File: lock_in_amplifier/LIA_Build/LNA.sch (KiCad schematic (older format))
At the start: 45 parts, among them J17 RF_Shield_One_Piece, J38 RF_Shield_One_Piece, U6 lmp7721, U7 LM833, U8 AD8429

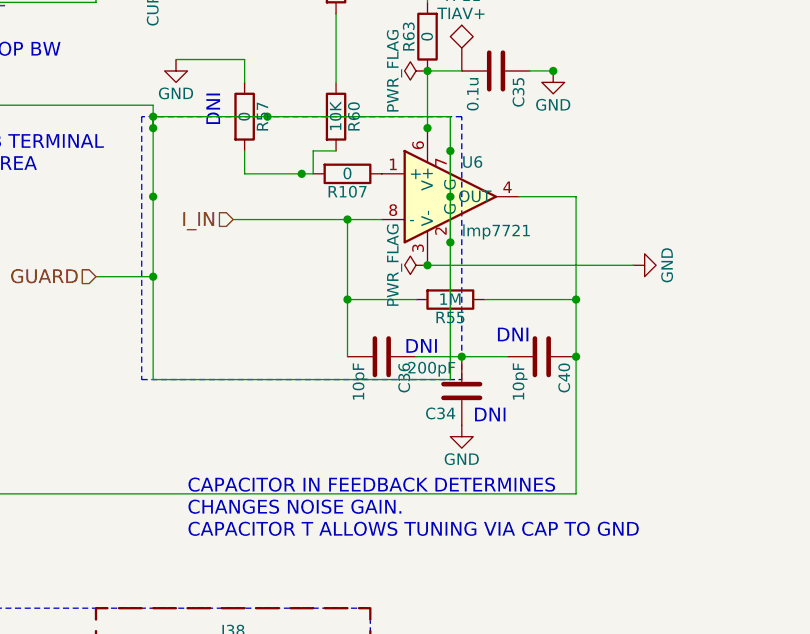
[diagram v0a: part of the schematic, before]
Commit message: adressing comments - fets
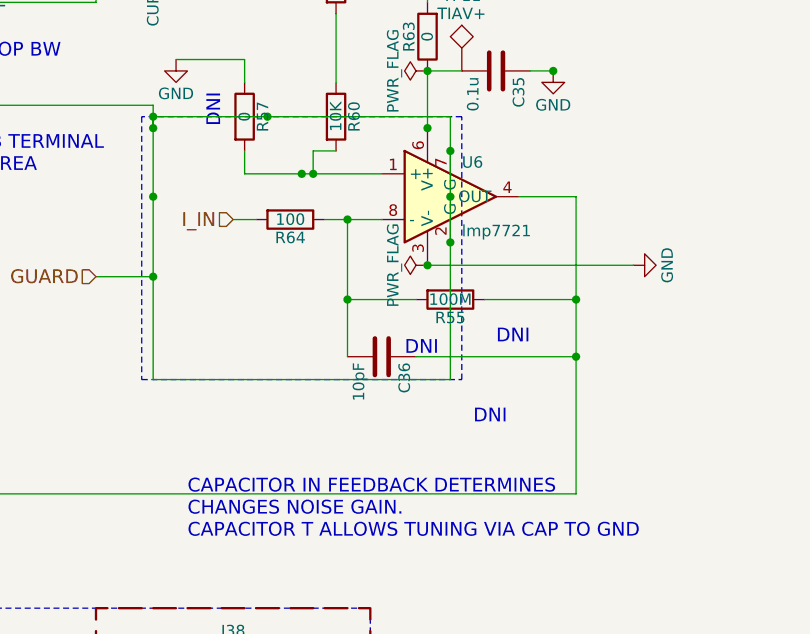
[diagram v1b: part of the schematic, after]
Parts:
- removed C34: 200pF, Capacitors_SMD:C_0805, symbol C
- removed C40: 10pF, Capacitors_SMD:C_0805, symbol C
- removed R107: 0, Resistors_SMD:R_0805, symbol R
- added R64: 100, Resistors_SMD:R_0805, symbol R
- R55: value 1M -> 100M
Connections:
- net I_IN: now also R64.2; no longer C36.2, R55.2, U6.8 (-)
- net at R55.1, S4.1 (B1), TP13.1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: now also C36.1
- net at R57.2, R60.2: now also U6.1 (+)
- new net: C36.2, R55.2, R64.1, U6.8 (-)
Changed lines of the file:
@@
 LIBS:contrib
 LIBS:valves
+LIBS:ada2200
 LIBS:LIA-cache
-LIBS:LNA_test-cache
 EELAYER 25 0
 EELAYER END
 $Descr USLetter 11000 8500
 encoding utf-8
-Sheet 3 3
+Sheet 3 6
 Title "LNA AND TRANSIMPEDANCE AMPLIFIER"
 Date ""
@@
 $EndComp
 $Comp
-L GND #PWR041
+L GND #PWR73
 U 1 1 5A1C75B0
 P 4100 7200
-F 0 "#PWR041" H 4100 6950 50  0001 C CNN
+F 0 "#PWR73" H 4100 6950 50  0001 C CNN
 F 1 "GND" H 4100 7050 50  0000 C CNN
 F 2 "" H 4100 7200 50  0001 C CNN
@@
 $EndComp
 $Comp
-L GND #PWR042
+L GND #PWR77
 U 1 1 5A1C75B6
 P 5100 5900
-F 0 "#PWR042" H 5100 5650 50  0001 C CNN
+F 0 "#PWR77" H 5100 5650 50  0001 C CNN
 F 1 "GND" H 5100 5750 50  0000 C CNN
 F 2 "" H 5100 5900 50  0001 C CNN
@@
 TRANSIMPEDANCE AMPLIFIER
 $Comp
-L GND #PWR043
+L GND #PWR71
 U 1 1 5A1F5BDB
 P 1450 6950
-F 0 "#PWR043" H 1450 6700 50  0001 C CNN
+F 0 "#PWR71" H 1450 6700 50  0001 C CNN
 F 1 "GND" H 1450 6800 50  0000 C CNN
 F 2 "" H 1450 6950 50  0001 C CNN
@@
 $EndComp
 $Comp
-L GND #PWR044
+L GND #PWR78
 U 1 1 5A276A01
 P 5750 6900
-F 0 "#PWR044" H 5750 6650 50  0001 C CNN
+F 0 "#PWR78" H 5750 6650 50  0001 C CNN
 F 1 "GND" H 5750 6750 50  0000 C CNN
 F 2 "" H 5750 6900 50  0001 C CNN
@@
 $EndComp
 $Comp
-L GND #PWR045
+L GND #PWR69
 U 1 1 5A277FAE
 P 1100 6050
-F 0 "#PWR045" H 1100 5800 50  0001 C CNN
+F 0 "#PWR69" H 1100 5800 50  0001 C CNN
 F 1 "GND" H 1100 5900 50  0000 C CNN
 F 2 "" H 1100 6050 50  0001 C CNN
@@
 $EndComp
 $Comp
-L GND #PWR046
+L GND #PWR70
 U 1 1 5A277FE0
 P 1200 7050
-F 0 "#PWR046" H 1200 6800 50  0001 C CNN
+F 0 "#PWR70" H 1200 6800 50  0001 C CNN
 F 1 "GND" H 1200 6900 50  0000 C CNN
 F 2 "" H 1200 7050 50  0001 C CNN
@@
 $EndComp
 $Comp
-L GND #PWR047
+L GND #PWR80
 U 1 1 5A21D13B
 P 6850 3300
-F 0 "#PWR047" H 6850 3050 50  0001 C CNN
+F 0 "#PWR80" H 6850 3050 50  0001 C CNN
 F 1 "GND" H 6850 3150 50  0000 C CNN
 F 2 "" H 6850 3300 50  0001 C CNN
@@
 $EndComp
 $Comp
-L GND #PWR048
+L GND #PWR79
 U 1 1 5A21D39E
 P 6500 2450
-F 0 "#PWR048" H 6500 2200 50  0001 C CNN
+F 0 "#PWR79" H 6500 2200 50  0001 C CNN
 F 1 "GND" H 6500 2300 50  0000 C CNN
 F 2 "" H 6500 2450 50  0001 C CNN
@@
 P 6050 3450
 F 0 "R55" V 6130 3450 50  0000 C CNN
-F 1 "1M" V 6050 3450 50  0000 C CNN
+F 1 "100M" V 6050 3450 50  0000 C CNN
 F 2 "Resistors_SMD:R_0805" V 5980 3450 50  0001 C CNN
 F 3 "" H 6050 3450 50  0001 C CNN
@@
 GUARD DRIVER
 $Comp
-L GND #PWR049
+L GND #PWR74
 U 1 1 5A220C69
 P 4200 1100
-F 0 "#PWR049" H 4200 850 50  0001 C CNN
+F 0 "#PWR74" H 4200 850 50  0001 C CNN
 F 1 "GND" H 4200 950 50  0000 C CNN
 F 2 "" H 4200 1100 50  0001 C CNN
@@
 +5v
 $Comp
-L GND #PWR050
+L GND #PWR75
 U 1 1 5A220E76
 P 4200 1800
-F 0 "#PWR050" H 4200 1550 50  0001 C CNN
+F 0 "#PWR75" H 4200 1550 50  0001 C CNN
 F 1 "GND" H 4200 1650 50  0000 C CNN
 F 2 "" H 4200 1800 50  0001 C CNN
@@
 $EndComp
 $Comp
-L GND #PWR051
+L GND #PWR72
 U 1 1 5A221F33
 P 1550 2900
-F 0 "#PWR051" H 1550 2650 50  0001 C CNN
+F 0 "#PWR72" H 1550 2650 50  0001 C CNN
 F 1 "GND" H 1550 2750 50  0000 C CNN
 F 2 "" H 1550 2900 50  0001 C CNN
@@
 DNI
 $Comp
-L GND #PWR052
+L GND #PWR76
 U 1 1 5A2235D5
 P 4850 2400
-F 0 "#PWR052" H 4850 2150 50  0001 C CNN
+F 0 "#PWR76" H 4850 2150 50  0001 C CNN
 F 1 "GND" H 4850 2250 50  0000 C CNN
 F 2 "" H 4850 2400 50  0001 C CNN
@@
 	1    0    0    -1
 $EndComp
-$Comp
-L C C40
-U 1 1 5A2420E6
-P 6450 3700
-F 0 "C40" H 6475 3800 50  0000 L CNN
-F 1 "10pF" H 6475 3600 50  0000 L CNN
-F 2 "Capacitors_SMD:C_0805" H 6488 3550 50  0001 C CNN
-F 3 "" H 6450 3700 50  0001 C CNN
-	1    6450 3700
-	0    1    1    0
-$EndComp
-$Comp
-L C C34
-U 1 1 5A2421FA
-P 6100 3850
-F 0 "C34" H 6125 3950 50  0000 L CNN
-F 1 "200pF" H 6125 3750 50  0000 L CNN
-F 2 "Capacitors_SMD:C_0805" H 6138 3700 50  0001 C CNN
-F 3 "" H 6100 3850 50  0001 C CNN
-	1    6100 3850
-	-1   0    0    1
-$EndComp
 Text Notes 6150 4000 0    60   ~ 0
 DNI
 Text Notes 6250 3650 0    60   ~ 0
 DNI
-$Comp
-L GND #PWR053
-U 1 1 5A2424BB
-P 6100 4000
-F 0 "#PWR053" H 6100 3750 50  0001 C CNN
-F 1 "GND" H 6100 3850 50  0000 C CNN
-F 2 "" H 6100 4000 50  0001 C CNN
-F 3 "" H 6100 4000 50  0001 C CNN
-	1    6100 4000
-	-1   0    0    -1
-$EndComp
 $Comp
 L R R63
@@
 Connection ~ 5250 2650
 Wire Wire Line
-	5100 3100 5750 3100
-Wire Wire Line
 	4750 2600 4750 3800
 Wire Wire Line
@@
 Connection ~ 6050 2800
 Wire Wire Line
-	5150 2900 5450 2900
+	5150 2900 5750 2900
 Connection ~ 4750 2650
 Connection ~ 1550 2600
@@
 Connection ~ 5250 1400
 Connection ~ 5400 2900
-Wire Wire Line
-	5900 3700 6300 3700
-Connection ~ 6100 3700
 Wire Wire Line
 	5950 3300 6850 3300
@@
 Connection ~ 3400 2050
 $Comp
-L PWR_FLAG #FLG054
+L PWR_FLAG #FLG9
 U 1 1 5A2D348D
 P 3650 1100
-F 0 "#FLG054" H 3650 1175 50  0001 C CNN
+F 0 "#FLG9" H 3650 1175 50  0001 C CNN
 F 1 "PWR_FLAG" H 3650 1250 50  0000 C CNN
 F 2 "" H 3650 1100 50  0001 C CNN
@@
 $EndComp
 $Comp
-L PWR_FLAG #FLG055
+L PWR_FLAG #FLG10
 U 1 1 5A2D35B5
 P 3650 1800
-F 0 "#FLG055" H 3650 1875 50  0001 C CNN
+F 0 "#FLG10" H 3650 1875 50  0001 C CNN
 F 1 "PWR_FLAG" H 3650 1950 50  0000 C CNN
 F 2 "" H 3650 1800 50  0001 C CNN
@@
 $EndComp
 $Comp
-L PWR_FLAG #FLG056
+L PWR_FLAG #FLG11
 U 1 1 5A2D36AF
 P 5950 2450
-F 0 "#FLG056" H 5950 2525 50  0001 C CNN
+F 0 "#FLG11" H 5950 2525 50  0001 C CNN
 F 1 "PWR_FLAG" H 5950 2600 50  0000 C CNN
 F 2 "" H 5950 2450 50  0001 C CNN
@@
 $EndComp
 $Comp
-L PWR_FLAG #FLG057
+L PWR_FLAG #FLG12
 U 1 1 5A2D374D
 P 5950 3300
-F 0 "#FLG057" H 5950 3375 50  0001 C CNN
+F 0 "#FLG12" H 5950 3375 50  0001 C CNN
 F 1 "PWR_FLAG" H 5950 3450 50  0000 C CNN
 F 2 "" H 5950 3300 50  0001 C CNN
@@
 	1    5950 3300
 	0    -1   -1   0
-$EndComp
-$Comp
-L R R107
-U 1 1 5A3351D4
-P 5600 2900
-F 0 "R107" V 5680 2900 50  0000 C CNN
-F 1 "0" V 5600 2900 50  0000 C CNN
-F 2 "Resistors_SMD:R_0805" V 5530 2900 50  0001 C CNN
-F 3 "" H 5600 2900 50  0001 C CNN
-	1    5600 2900
-	0    1    1    0
 $EndComp
 Wire Wire Line
@@
 Wire Wire Line
 	5550 1400 5550 1900
+$Comp
+L R R64
+U 1 1 5A3975B2
+P 5350 3100
+F 0 "R64" V 5430 3100 50  0000 C CNN
+F 1 "100" V 5350 3100 50  0000 C CNN
+F 2 "Resistors_SMD:R_0805" V 5280 3100 50  0001 C CNN
+F 3 "" H 5350 3100 50  0001 C CNN
+	1    5350 3100
+	0    1    1    0
+$EndComp
+Wire Wire Line
+	5100 3100 5200 3100
+Wire Wire Line
+	5500 3100 5750 3100
+Wire Wire Line
+	5900 3700 6600 3700
+Connection ~ 5450 2900
 $EndSCHEMATC
